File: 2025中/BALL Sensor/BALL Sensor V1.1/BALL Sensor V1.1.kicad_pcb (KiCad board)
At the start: 2 copper layers, 100 x 100 mm, 43 parts, among them J1 Conn_02x04_Odd_Even, J2 Conn_01x05_Pin, SW2 SW_MEC_5G, U2 ATmega32U4-A, Y1 CSTCE16M0V53-R0

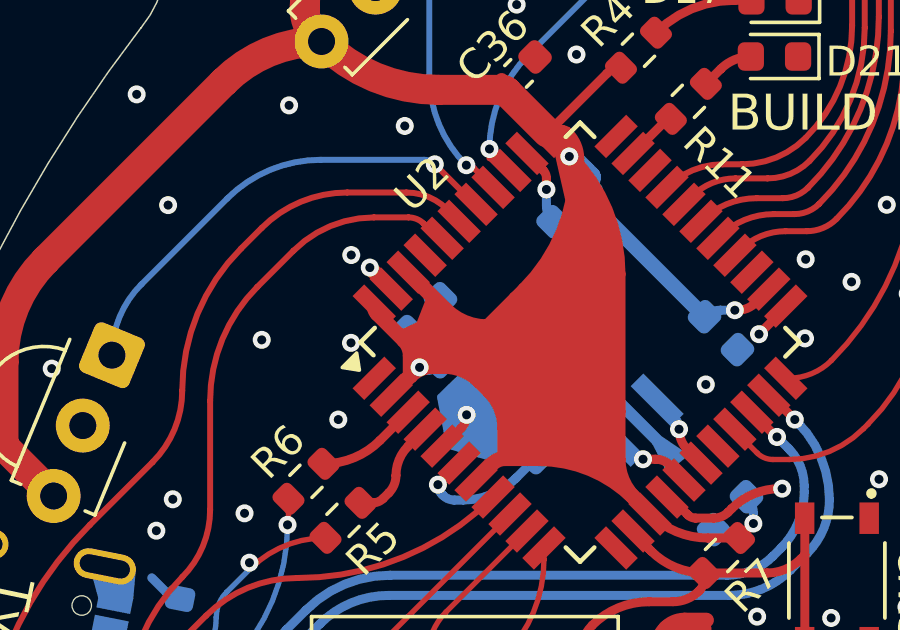
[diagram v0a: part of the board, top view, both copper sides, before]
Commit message: 定期更新
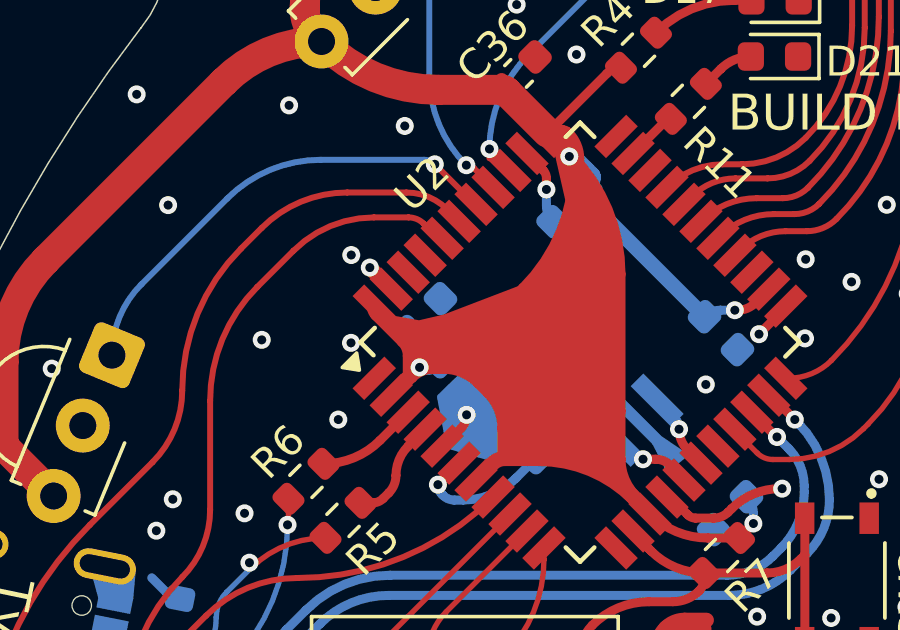
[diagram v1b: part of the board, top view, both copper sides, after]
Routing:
- net +5V: track 378.5 -> 375.2 mm
